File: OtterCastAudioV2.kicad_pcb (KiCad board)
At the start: 4 copper layers, 50 x 49.3 mm, 229 parts, among them J1 UART, J2 SD, J3 USB, J4 OTG, J5 PJ-3270, J6 PJ-3270, J7 PJ-3270, J8 49F-1201GYD2NL, Q1 DTA114YKA, SW3 RST, U1 AllWinner-S3(FBGA-234), U3 AXP209(QFN-48), U4 SY8089AAAC, U5 SY6280AAC, U6 SSM2603, U7 AP6236, X1 26Mhz TCXO, Y1 12.288Mhz, Y2 32.768kHz, Y3 24MHz

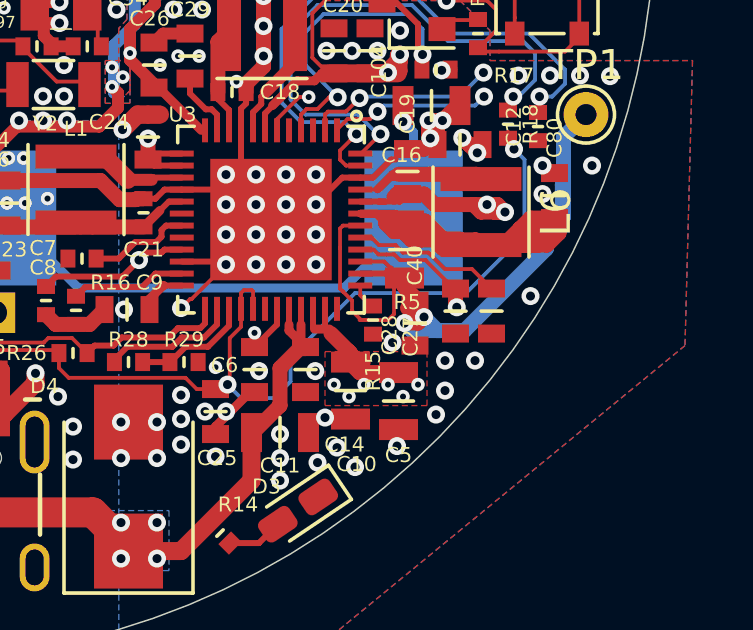
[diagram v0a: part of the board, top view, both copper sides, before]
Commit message: Improce IPS connectivity
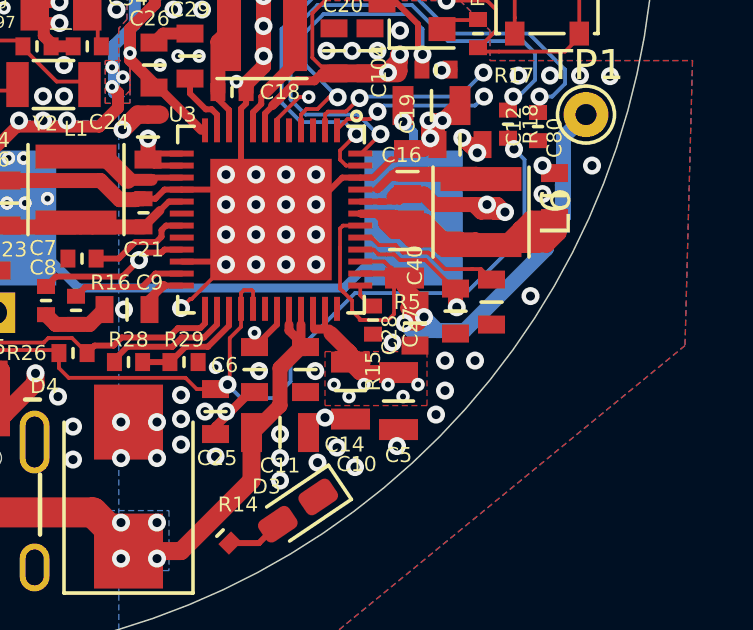
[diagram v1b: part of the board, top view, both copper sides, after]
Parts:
- moved C27 0.30 mm to (119.5, 113.0)
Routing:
- net IPS: track 114.6 -> 126.8 mm
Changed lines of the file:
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@@
     (thickness 1.6)
     (drawings 70)
-    (tracks 3443)
+    (tracks 3477)
     (zones 0)
     (modules 229)
@@
   )
   (module otter:C_0603 (layer F.Cu)
-    (at 119.55 113.35 270)
+    (at 119.55 113.05 270)
     (descr "Capacitor 0603")
     (tags "C Capacitor 0603")
@@
   (segment (start 108.1 107.6) (end 110.901065 107.6) (width 0.5) (layer In1.Cu) (net 6))
   (segment (start 110.901065 107.6) (end 113.124576 105.376489) (width 0.5) (layer In1.Cu) (net 6))
-  (segment (start 113.124576 105.376489) (end 116.376489 105.376489) (width 0.5) (layer In1.Cu) (net 6))
   (segment (start 116.376489 105.376489) (end 116.5 105.5) (width 0.5) (layer In1.Cu) (net 6))
   (segment (start 119.25 107.9) (end 119.075 108.075) (width 0.5) (layer F.Cu) (net 6))
@@
   (segment (start 118.575 107.575) (end 118.575 106.325) (width 0.5) (layer In1.Cu) (net 6))
   (segment (start 118.575 106.325) (end 118.3 106.05) (width 0.5) (layer In1.Cu) (net 6))
-  (segment (start 117.05 106.05) (end 116.5 105.5) (width 0.5) (layer In1.Cu) (net 6))
   (segment (start 118.3 106.05) (end 117.05 106.05) (width 0.5) (layer In1.Cu) (net 6))
   (segment (start 116.55 115.4) (end 115.15 115.4) (width 0.5) (layer F.Cu) (net 6))
@@
   (segment (start 117.35 111.65) (end 118.35 112.65) (width 0.127) (layer F.Cu) (net 6))
   (segment (start 118.35 112.65) (end 118.4 112.65) (width 0.127) (layer F.Cu) (net 6))
-  (segment (start 116.1 115.8) (end 118.4 113.5) (width 0.5) (layer In1.Cu) (net 6))
   (segment (start 118.4 113.5) (end 118.35 113.5) (width 0.5) (layer In1.Cu) (net 6))
   (segment (start 118.35 113.18165) (end 118.39185 113.2235) (width 0.5) (layer F.Cu) (net 6))
@@
   (via (at 118.39185 113.2235) (size 0.6) (drill 0.3) (layers F.Cu B.Cu) (net 6))
   (segment (start 119.075 108.075) (end 119.4 108.4) (width 0.5) (layer In1.Cu) (net 6))
-  (segment (start 119.4 112.21535) (end 118.39185 113.2235) (width 0.5) (layer In1.Cu) (net 6))
   (via (at 119.4 109.8) (size 0.6) (drill 0.3) (layers F.Cu B.Cu) (net 6))
-  (segment (start 119.4 108.4) (end 119.4 109.8) (width 0.5) (layer In1.Cu) (net 6))
   (via (at 120 110.05) (size 0.6) (drill 0.3) (layers F.Cu B.Cu) (net 6))
   (segment (start 119.75 109.8) (end 120 110.05) (width 0.5) (layer In1.Cu) (net 6))
@@
   (segment (start 116.2 105.5) (end 116.1 105.4) (width 0.5) (layer In1.Cu) (net 6))
   (segment (start 116.5 105.5) (end 116.2 105.5) (width 0.5) (layer In1.Cu) (net 6))
+  (segment (start 118.575 107.575) (end 119.025 107.575) (width 0.5) (layer In1.Cu) (net 6))
+  (segment (start 119.025 107.575) (end 119.55 108.1) (width 0.5) (layer In1.Cu) (net 6))
+  (segment (start 119.55 108.25) (end 119.4 108.4) (width 0.5) (layer In1.Cu) (net 6))
+  (segment (start 119.55 108.1) (end 119.55 108.25) (width 0.5) (layer In1.Cu) (net 6))
+  (segment (start 119.55 108.25) (end 118.8 108.25) (width 0.5) (layer In1.Cu) (net 6))
+  (segment (start 118.8 108.25) (end 118.35 107.8) (width 0.5) (layer In1.Cu) (net 6))
+  (segment (start 118.35 107.8) (end 118.575 107.575) (width 0.5) (layer In1.Cu) (net 6))
+  (segment (start 118.35 107.8) (end 118.35 107.541802) (width 0.5) (layer In1.Cu) (net 6))
+  (segment (start 119.025 107.575) (end 119.025 107.325) (width 0.5) (layer In1.Cu) (net 6))
+  (segment (start 119.025 107.325) (end 118.85 107.15) (width 0.5) (layer In1.Cu) (net 6))
+  (segment (start 119.4 110.3) (end 119.3 110.3) (width 0.5) (layer In1.Cu) (net 6))
+  (segment (start 119.3 110.3) (end 119.05 110.05) (width 0.5) (layer In1.Cu) (net 6))
+  (segment (start 119.05 109.4) (end 119.4 109.05) (width 0.5) (layer In1.Cu) (net 6))
+  (segment (start 119.05 110.05) (end 119.05 109.4) (width 0.5) (layer In1.Cu) (net 6))
+  (segment (start 119.4 109.05) (end 119.4 109.8) (width 0.5) (layer In1.Cu) (net 6))
+  (segment (start 119.4 108.4) (end 119.4 109.05) (width 0.5) (layer In1.Cu) (net 6))
+  (segment (start 120 110.05) (end 120 110.4) (width 0.5) (layer In1.Cu) (net 6))
+  (segment (start 120 110.4) (end 119.8 110.6) (width 0.5) (layer In1.Cu) (net 6))
+  (segment (start 120 110.05) (end 120 109.55) (width 0.5) (layer In1.Cu) (net 6))
+  (segment (start 120 109.55) (end 119.75 109.3) (width 0.5) (layer In1.Cu) (net 6))
+  (segment (start 119.4 112.5) (end 118.4 113.5) (width 0.5) (layer In1.Cu) (net 6))
+  (segment (start 119.4 112.21535) (end 119.4 112.5) (width 0.5) (layer In1.Cu) (net 6))
+  (segment (start 118.125 113.49035) (end 118.39185 113.2235) (width 0.5) (layer In1.Cu) (net 6))
+  (segment (start 118.125 113.775) (end 118.125 113.49035) (width 0.5) (layer In1.Cu) (net 6))
+  (segment (start 116.1 115.8) (end 118.125 113.775) (width 0.5) (layer In1.Cu) (net 6))
+  (segment (start 118.275 113.625) (end 117.95 113.3) (width 0.5) (layer In1.Cu) (net 6))
+  (segment (start 118.125 113.775) (end 118.275 113.625) (width 0.5) (layer In1.Cu) (net 6))
+  (segment (start 118.275 113.625) (end 118.4 113.5) (width 0.5) (layer In1.Cu) (net 6))
+  (segment (start 118.367325 112.882675) (end 118.732675 112.882675) (width 0.5) (layer In1.Cu) (net 6))
+  (segment (start 117.95 113.3) (end 118.367325 112.882675) (width 0.5) (layer In1.Cu) (net 6))
+  (segment (start 118.732675 112.882675) (end 118.39185 113.2235) (width 0.5) (layer In1.Cu) (net 6))
+  (segment (start 119.4 112.21535) (end 118.732675 112.882675) (width 0.5) (layer In1.Cu) (net 6))
+  (segment (start 115.9 105.75) (end 115.526489 105.376489) (width 0.5) (layer In1.Cu) (net 6))
+  (segment (start 116.75 105.75) (end 115.9 105.75) (width 0.5) (layer In1.Cu) (net 6))
+  (segment (start 115.526489 105.376489) (end 116.376489 105.376489) (width 0.5) (layer In1.Cu) (net 6))
+  (segment (start 113.124576 105.376489) (end 115.526489 105.376489) (width 0.5) (layer In1.Cu) (net 6))
+  (segment (start 117.05 106.05) (end 116.75 105.75) (width 0.5) (layer In1.Cu) (net 6))
+  (segment (start 116.75 105.75) (end 116.5 105.5) (width 0.5) (layer In1.Cu) (net 6))
   (via (at 91.325 115.8) (size 0.45) (drill 0.2) (layers F.Cu B.Cu) (net 7))
   (segment (start 112.4 113.8) (end 111.65 114.55) (width 0.2) (layer F.Cu) (net 7))
@@
   (segment (start 118.9 111.95) (end 118 111.95) (width 0.127) (layer F.Cu) (net 15))
   (segment (start 115.552516 110.9) (end 115.175 110.9) (width 0.127) (layer F.Cu) (net 15))
-  (segment (start 119.55 112.6) (end 118.9 111.95) (width 0.127) (layer F.Cu) (net 15))
+  (segment (start 118.9 111.95) (end 119.2 111.95) (width 0.127) (layer F.Cu) (net 15))
+  (segment (start 119.2 111.95) (end 119.55 112.3) (width 0.127) (layer F.Cu) (net 15))
   (segment (start 109.5 106.1) (end 109.5 105.6) (width 0.2) (layer F.Cu) (net 16))
   (segment (start 110.025 106.625) (end 109.5 106.1) (width 0.2) (layer F.Cu) (net 16))
